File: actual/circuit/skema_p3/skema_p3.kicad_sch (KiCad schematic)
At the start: 0 parts

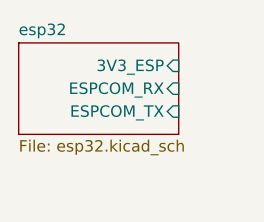
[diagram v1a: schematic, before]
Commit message: P3 in KiCAD
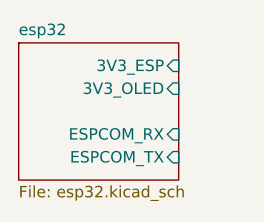
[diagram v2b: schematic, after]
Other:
- sheet esp32 ports: added 3V3_OLED; removed none
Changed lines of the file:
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@@
 (kicad_sch (version 20211123) (generator eeschema)
   (paper "A4")
-  (sheet (at 39.37 27.94) (size 17.78 10.16) (fields_autoplaced)
+  (sheet (at 39.37 27.94) (size 17.78 15.24) (fields_autoplaced)
     (stroke (width 0.1524) (type solid) (color 0 0 0 0))
     (fill (color 0 0 0 0.0000))
@@
       (effects (font (size 1.27 1.27)) (justify left bottom))
     )
-    (property "Sheet file" "esp32.kicad_sch" (id 1) (at 39.37 38.6846 0)
+    (property "Sheet file" "esp32.kicad_sch" (id 1) (at 39.37 43.7646 0)
       (effects (font (size 1.27 1.27)) (justify left top))
     )
@@
       (effects (font (size 1.27 1.27)) (justify right))
     )
-    (pin "ESPCOM_RX" input (at 57.15 33.02 0)
+    (pin "ESPCOM_RX" input (at 57.15 38.1 0)
       (effects (font (size 1.27 1.27)) (justify right))
     )
-    (pin "ESPCOM_TX" input (at 57.15 35.56 0)
+    (pin "ESPCOM_TX" input (at 57.15 40.64 0)
+      (effects (font (size 1.27 1.27)) (justify right))
+    )
+    (pin "3V3_OLED" input (at 57.15 33.02 0)
       (effects (font (size 1.27 1.27)) (justify right))
     )
@@
       (reference "#PWR04") (unit 1) (value "GND") (footprint "")
     )
+    (path "/597d0667-4207-4756-9f1e-dc2b80c39ef1/4dcd3d3a-119a-44da-9b9d-811f366562de"
+      (reference "#PWR05") (unit 1) (value "GND") (footprint "")
+    )
+    (path "/597d0667-4207-4756-9f1e-dc2b80c39ef1/51f570fc-c5f7-4af1-b862-d3ce48e1897c"
+      (reference "#PWR06") (unit 1) (value "GND") (footprint "")
+    )
+    (path "/597d0667-4207-4756-9f1e-dc2b80c39ef1/3fb3901e-83b5-4621-989d-017e7f512a09"
+      (reference "#PWR07") (unit 1) (value "GND") (footprint "")
+    )
+    (path "/597d0667-4207-4756-9f1e-dc2b80c39ef1/04552b8c-f119-473d-a0a5-d16c45a3d21b"
+      (reference "#PWR08") (unit 1) (value "GND") (footprint "")
+    )
+    (path "/597d0667-4207-4756-9f1e-dc2b80c39ef1/6c861eee-6fd4-4fd4-8e25-748796aa0d0a"
+      (reference "#PWR09") (unit 1) (value "GND") (footprint "")
+    )
+    (path "/597d0667-4207-4756-9f1e-dc2b80c39ef1/9a18e0a8-054a-4d5d-aa0d-dd1c17bbb27e"
+      (reference "#PWR010") (unit 1) (value "GND") (footprint "")
+    )
+    (path "/597d0667-4207-4756-9f1e-dc2b80c39ef1/05699855-e787-4748-b5c1-d54464eb2c0f"
+      (reference "#PWR011") (unit 1) (value "GND") (footprint "")
+    )
+    (path "/597d0667-4207-4756-9f1e-dc2b80c39ef1/35709dbc-6113-4681-a2fe-9607a1e10ff5"
+      (reference "Brd1") (unit 1) (value "SSD1306") (footprint "")
+    )
     (path "/597d0667-4207-4756-9f1e-dc2b80c39ef1/bf848998-97a4-4380-99f3-b2742573bde0"
       (reference "C1") (unit 1) (value "100uF") (footprint "")
+    )
+    (path "/597d0667-4207-4756-9f1e-dc2b80c39ef1/8fb303f9-220f-48ae-9073-3c8ea3ed7281"
+      (reference "C2") (unit 1) (value "4.7uF") (footprint "")
+    )
+    (path "/597d0667-4207-4756-9f1e-dc2b80c39ef1/0d1b0445-a1ea-4320-92e8-9c7aaca19265"
+      (reference "C3") (unit 1) (value "4.7uF") (footprint "")
+    )
+    (path "/597d0667-4207-4756-9f1e-dc2b80c39ef1/f869e314-79cf-403e-b735-bc4b7a5e67c4"
+      (reference "C4") (unit 1) (value "4.7uF") (footprint "")
+    )
+    (path "/597d0667-4207-4756-9f1e-dc2b80c39ef1/aecbee31-7d90-4cd5-ae31-9903b210c381"
+      (reference "C5") (unit 1) (value "22pF") (footprint "")
+    )
+    (path "/597d0667-4207-4756-9f1e-dc2b80c39ef1/bceaa45a-0015-46f9-be94-d75ebaa21cd8"
+      (reference "C6") (unit 1) (value "22pF") (footprint "")
+    )
+    (path "/597d0667-4207-4756-9f1e-dc2b80c39ef1/8e958225-40e7-4ae6-9bd6-c92bea46fb51"
+      (reference "C7") (unit 1) (value "4.7uF") (footprint "")
     )
     (path "/597d0667-4207-4756-9f1e-dc2b80c39ef1/053eb1c6-8a54-44cc-bb35-25e43aeee1de"
@@
       (reference "R8") (unit 1) (value "0") (footprint "")
     )
+    (path "/597d0667-4207-4756-9f1e-dc2b80c39ef1/4222ebfe-27d9-4f84-8800-1e1f780b4e08"
+      (reference "R9") (unit 1) (value "10K") (footprint "")
+    )
+    (path "/597d0667-4207-4756-9f1e-dc2b80c39ef1/54c4d94b-9fb0-43fd-943b-199d31e7c4a2"
+      (reference "R10") (unit 1) (value "10K") (footprint "")
+    )
+    (path "/597d0667-4207-4756-9f1e-dc2b80c39ef1/8ae99862-332c-4ee4-9c32-81ff36f98d30"
+      (reference "R11") (unit 1) (value "10K") (footprint "")
+    )
+    (path "/597d0667-4207-4756-9f1e-dc2b80c39ef1/4a578110-80ff-4246-9d96-0515e0099dab"
+      (reference "R12") (unit 1) (value "10K") (footprint "")
+    )
+    (path "/597d0667-4207-4756-9f1e-dc2b80c39ef1/b1fb259f-b78c-4cb6-baf5-e0ac7b725924"
+      (reference "R13") (unit 1) (value "10K") (footprint "")
+    )
+    (path "/597d0667-4207-4756-9f1e-dc2b80c39ef1/9f8aad5b-f7d2-4724-874e-7c0d9eae25ae"
+      (reference "R14") (unit 1) (value "1K") (footprint "")
+    )
+    (path "/597d0667-4207-4756-9f1e-dc2b80c39ef1/aabfbc33-ba51-4fb9-b9ec-75b47f1bd138"
+      (reference "R15") (unit 1) (value "1K") (footprint "")
+    )
+    (path "/597d0667-4207-4756-9f1e-dc2b80c39ef1/d3f9a4d9-fa0e-41e8-8eab-8584088db3a6"
+      (reference "R16") (unit 1) (value "0") (footprint "")
+    )
+    (path "/597d0667-4207-4756-9f1e-dc2b80c39ef1/87119be6-3888-407e-976f-44367c5113e4"
+      (reference "SW1") (unit 1) (value "SW_Push") (footprint "")
+    )
+    (path "/597d0667-4207-4756-9f1e-dc2b80c39ef1/3852f08c-d658-4f28-80f2-b12717f261fd"
+      (reference "SW2") (unit 1) (value "SW_Push") (footprint "")
+    )
+    (path "/597d0667-4207-4756-9f1e-dc2b80c39ef1/cb3a121e-5a5a-4de0-8358-015431cb75c7"
+      (reference "SW3") (unit 1) (value "SW_Push") (footprint "")
+    )
+    (path "/597d0667-4207-4756-9f1e-dc2b80c39ef1/bf4ea66f-3529-4ecb-a4a7-247651409599"
+      (reference "SW4") (unit 1) (value "SW_Push") (footprint "")
+    )
+    (path "/597d0667-4207-4756-9f1e-dc2b80c39ef1/c5b69453-7cd9-4d3e-ac8e-835565cfca87"
+      (reference "SW5") (unit 1) (value "SW_Push") (footprint "")
+    )
     (path "/597d0667-4207-4756-9f1e-dc2b80c39ef1/4b0c433c-9d35-4622-81fa-d89b3e11d04a"
